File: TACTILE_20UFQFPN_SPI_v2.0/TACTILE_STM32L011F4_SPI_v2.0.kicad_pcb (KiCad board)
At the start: 2 copper layers, 20 x 32 mm, 24 parts, among them U2 DRV5057A1QDBZR, U3 DRV5057A1QDBZR, U4 DRV5057A1QDBZR, U5 DRV5057A1QDBZR

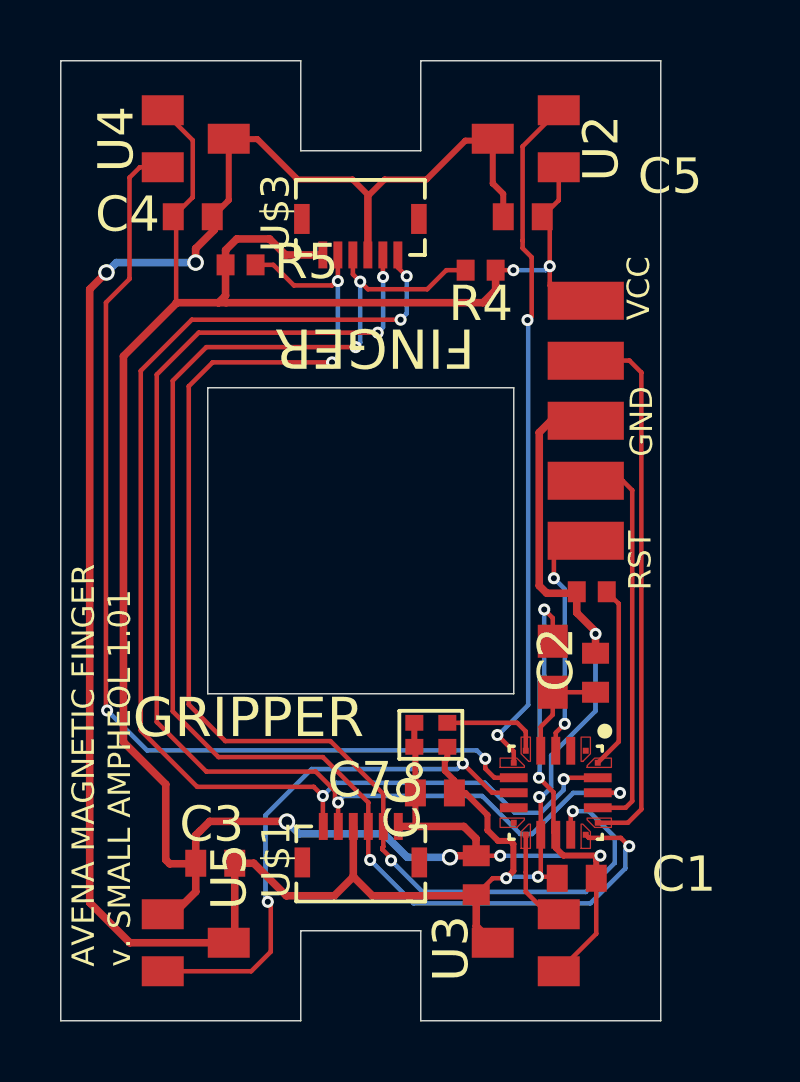
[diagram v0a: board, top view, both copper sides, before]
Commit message: update tactile pcb v2.0
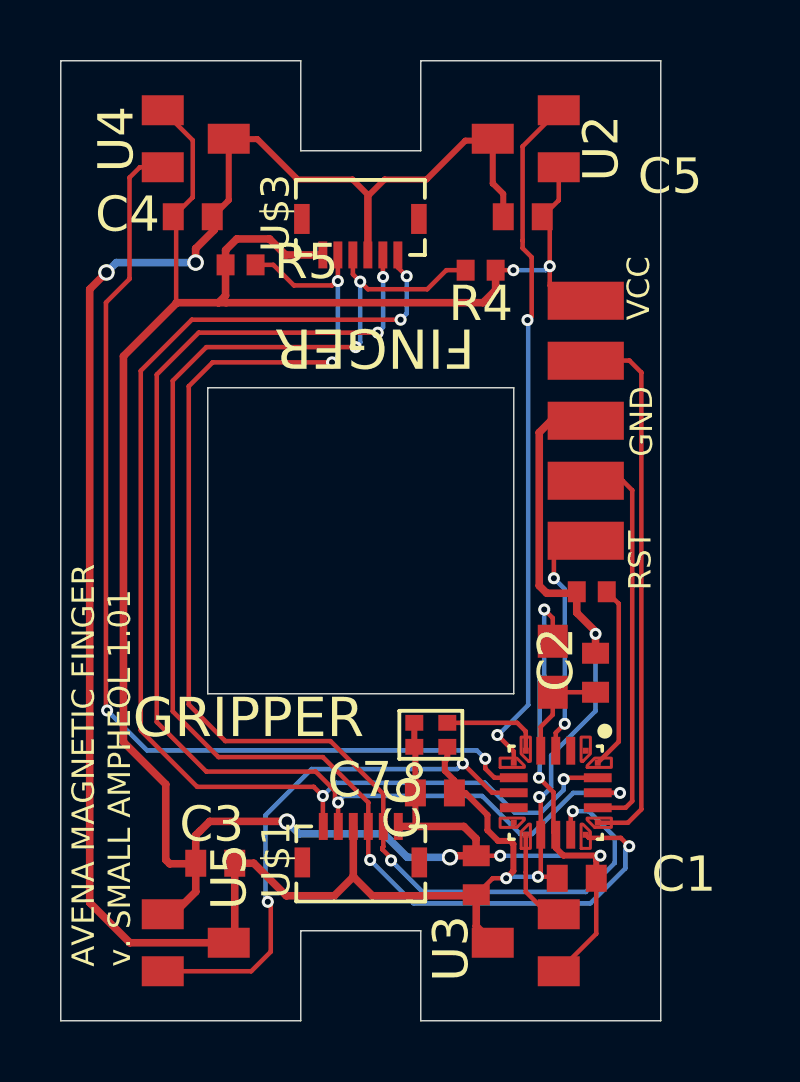
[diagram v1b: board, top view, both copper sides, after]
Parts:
- U2, U3, U4, U5: value DRV5057A1QDBZR -> DRV5056A4
